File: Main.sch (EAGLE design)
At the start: 40 parts, among them J1 USB-A1HSW6, U5 TP4056, U6 MT3608, U7 DS3231S, U8 AMS1117-3.3

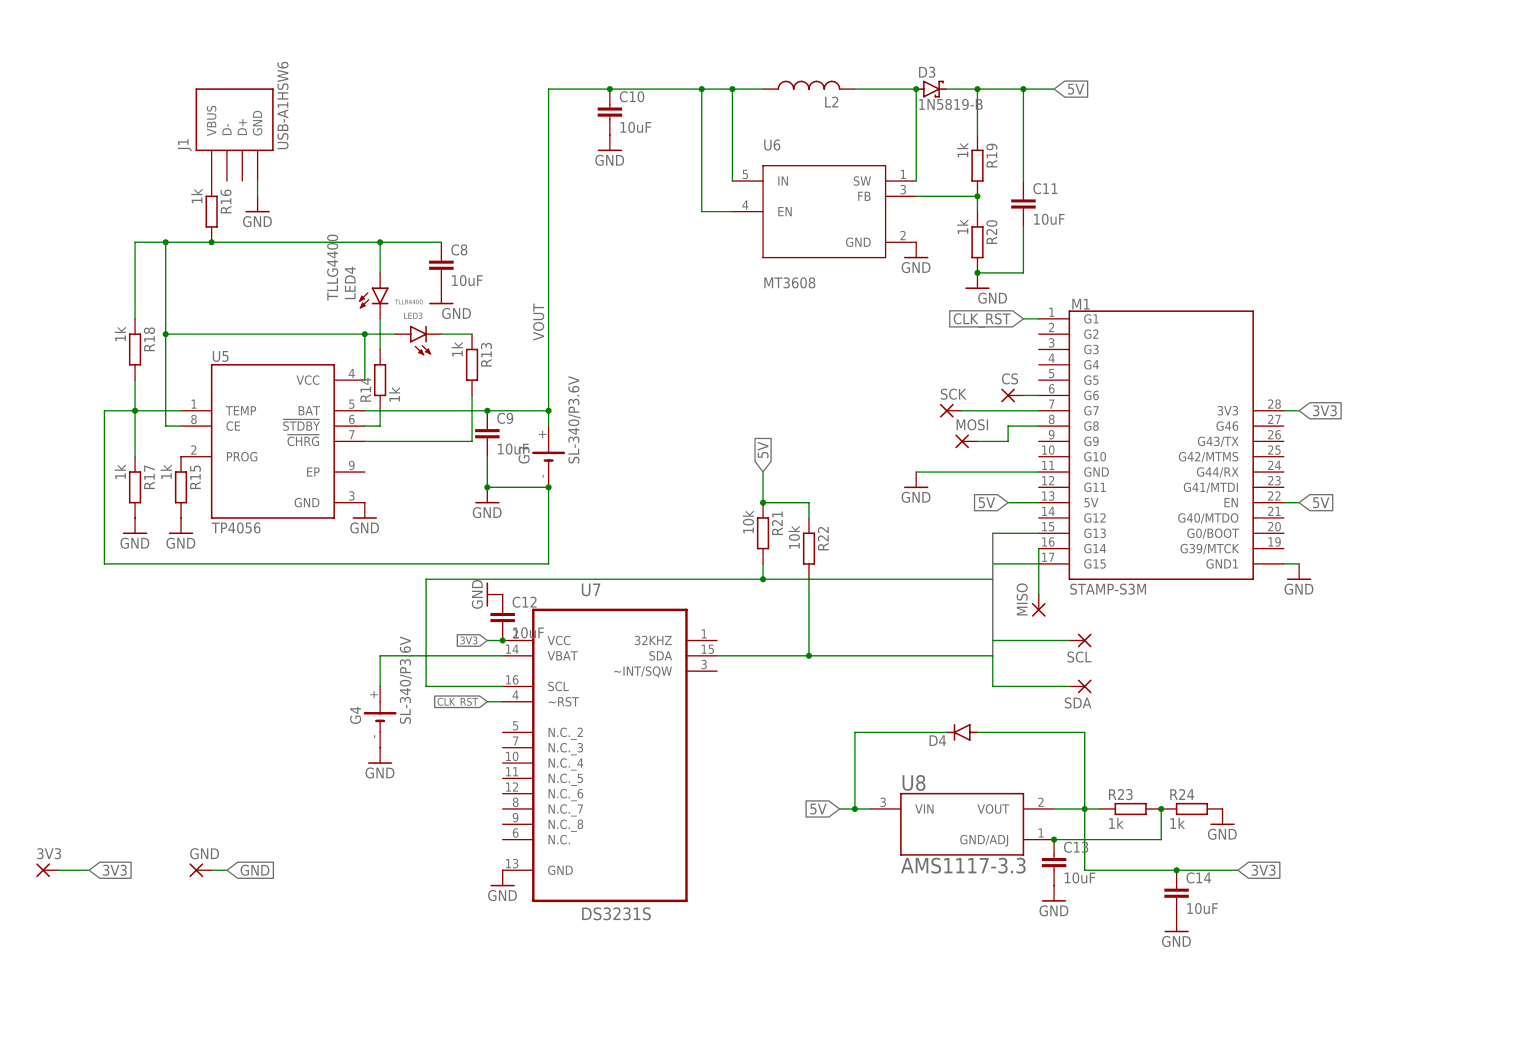
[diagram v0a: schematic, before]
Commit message: Add final project of PCB boards and cleaning repository up
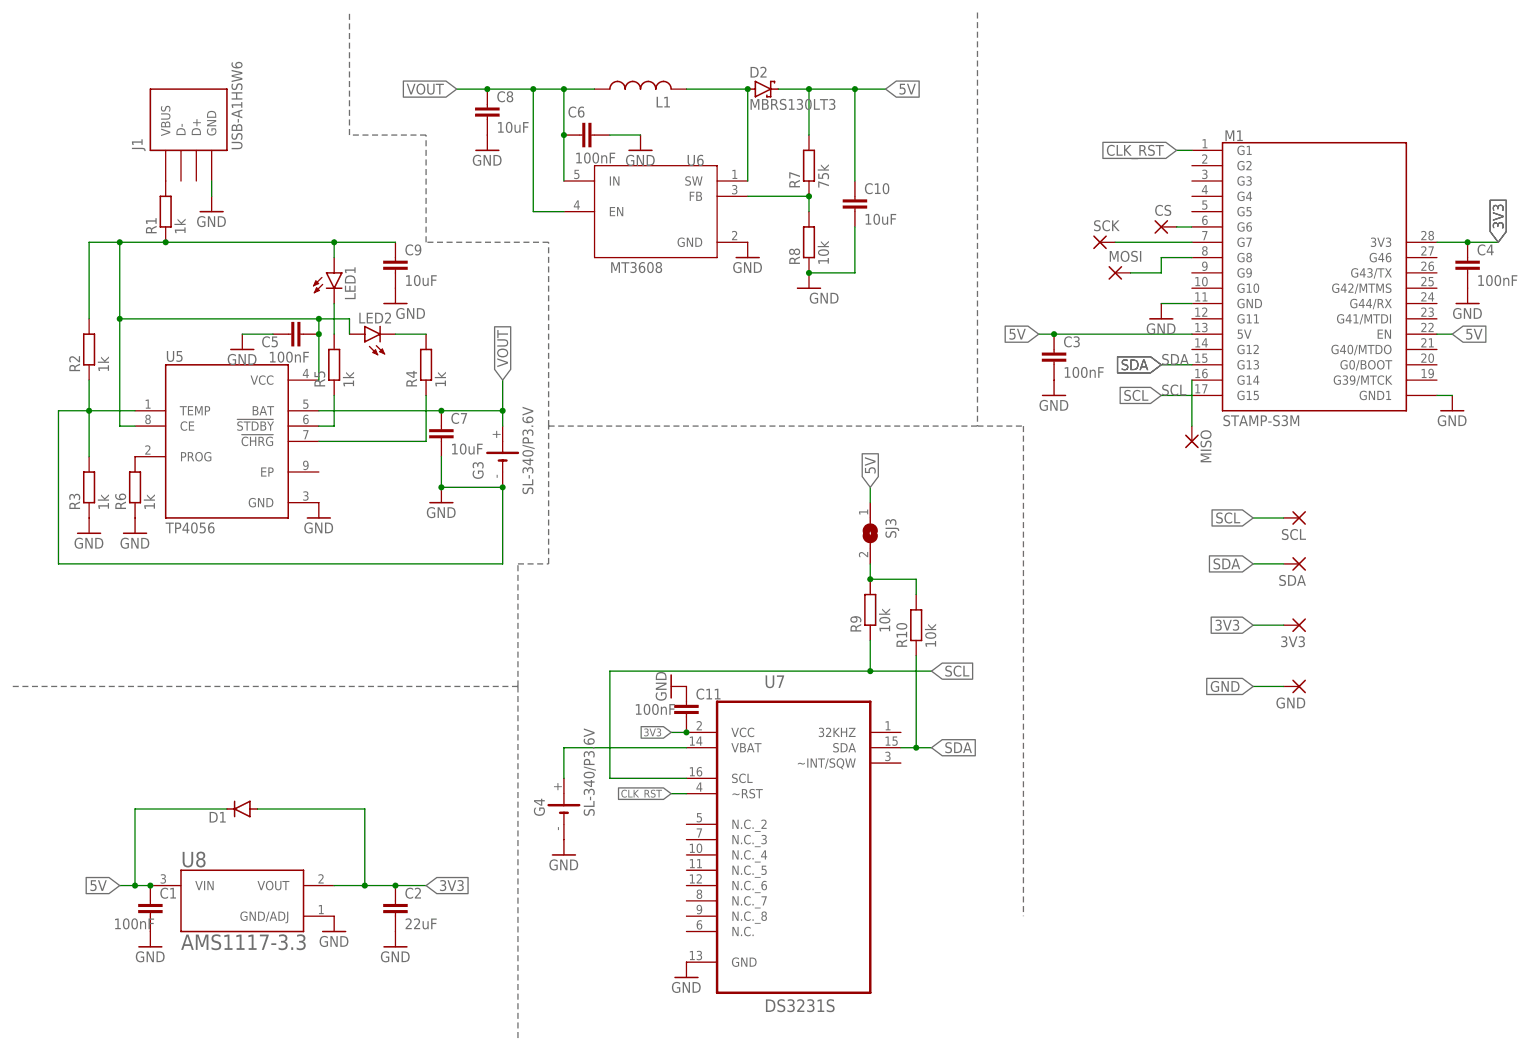
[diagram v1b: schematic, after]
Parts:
- removed C12, C13, C14: 10uF, capacitor-wima:C2,5-3
- removed D3: 1N5819-B, diode:1N5819-B
- removed D4: (no value), diode:DIODE-D-2.5
- removed L2: (no value), rcl:L-US0204/7
- removed LED3: TLLR4400, led:TLLR4400
- removed LED4: TLLG4400, led:TLLG4400
- removed R13, R14, R15, R16, R17, R18, R19, R20, R23, R24: 1k, rcl:R-EU_0204/2V
- removed R21, R22: 10k, rcl:R-EU_0204/2V
- added C1, C3, C4, C5, C6: 100nF, rcl:C-EUC0402
- added C2: 22uF, rcl:C-EUC0402
- added C7: 10uF, rcl:C-EUC0402
- added D1: (no value), diode:DIODE-SMB
- added D2: MBRS130LT3, diode:MBRS130LT3
- added L1: (no value), rcl:L-USL3225M
- added LED1, LED2: (no value), led:LEDCHIPLED_0805
- added R1, R2, R3, R4, R5, R6: 1k, rcl:R-EU_M1206
- added R10, R8, R9: 10k, rcl:R-EU_M1206
- added R7: 75k, rcl:R-EU_M1206
- added SJ3: (no value), jumper:SJ
- C10, C8, C9: device capacitor-wima:C2,5-3 -> rcl:C-EUC0402
- C11: value 10uF -> 100nF; device capacitor-wima:C2,5-3 -> rcl:C-EUC0402
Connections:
- removed net N$13: LED4.C, R14.2
- removed net N$14: LED3.C, R13.1
- removed net N$20: C13.1, R23.2, R24.1, U8.GND/ADJ
- new net CHRG2: LED2.C, R4.2
- new net JUMPER: R10.2, R9.2, SJ3.2
- new net N$2: LED1.C, R5.2
- new net N$3: J1.VBUS, R1.2
- net 3V3: now also C11.2, C2.1, C4.1, D1.A; no longer C12.2, C14.1, D4.A, R23.1
- net 5V: now also C1.1, C10.1, C3.1, D1.C, D2.C, R7.2, SJ3.1; no longer C11.1, D3.C, D4.C, R19.1, R21.1, R22.1
- net CHRG: now also R4.1; no longer R13.2
- net FB: now also R7.1, R8.2; no longer R19.2, R20.1
- net GND: now also C1.2, C11.1, C2.2, C3.2, C4.2, C5.1, C6.2, C7.2, R2.1, R3.1, R3.2, R6.1, R8.1, U8.GND/ADJ; no longer C11.2, C12.1, C13.2, C14.2, R15.2, R17.1, R17.2, R18.2, R20.2, R24.2
- net N$1: now also R6.2; no longer R15.1
- net SCL: now also R9.1; no longer R21.2
- net SDA: now also R10.1; no longer R22.2
- net STDBY: now also R5.1; no longer R14.1
- net SW: now also D2.A, L1.2; no longer D3.A, L2.2
- net USB1: now also C5.2, C9.1, LED1.A, LED2.A, R1.1, R2.2; no longer C8.1, J1.VBUS, LED3.A, LED4.A, R16.1, R16.2, R18.1
- net VOUT: now also C6.1, C7.1, C8.1, L1.1; no longer C10.1, C9.1, L2.1
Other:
- moved on the sheet: 3V3, C10, C11, C8, C9, CS, G3, G4, GND, J1, MISO, MOSI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
